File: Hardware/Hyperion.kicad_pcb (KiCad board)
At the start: 2 copper layers, 90.2 x 95.9 mm, 14 parts, among them J1 CUBESAT-BUS, U1 TM4C123GH6PZ

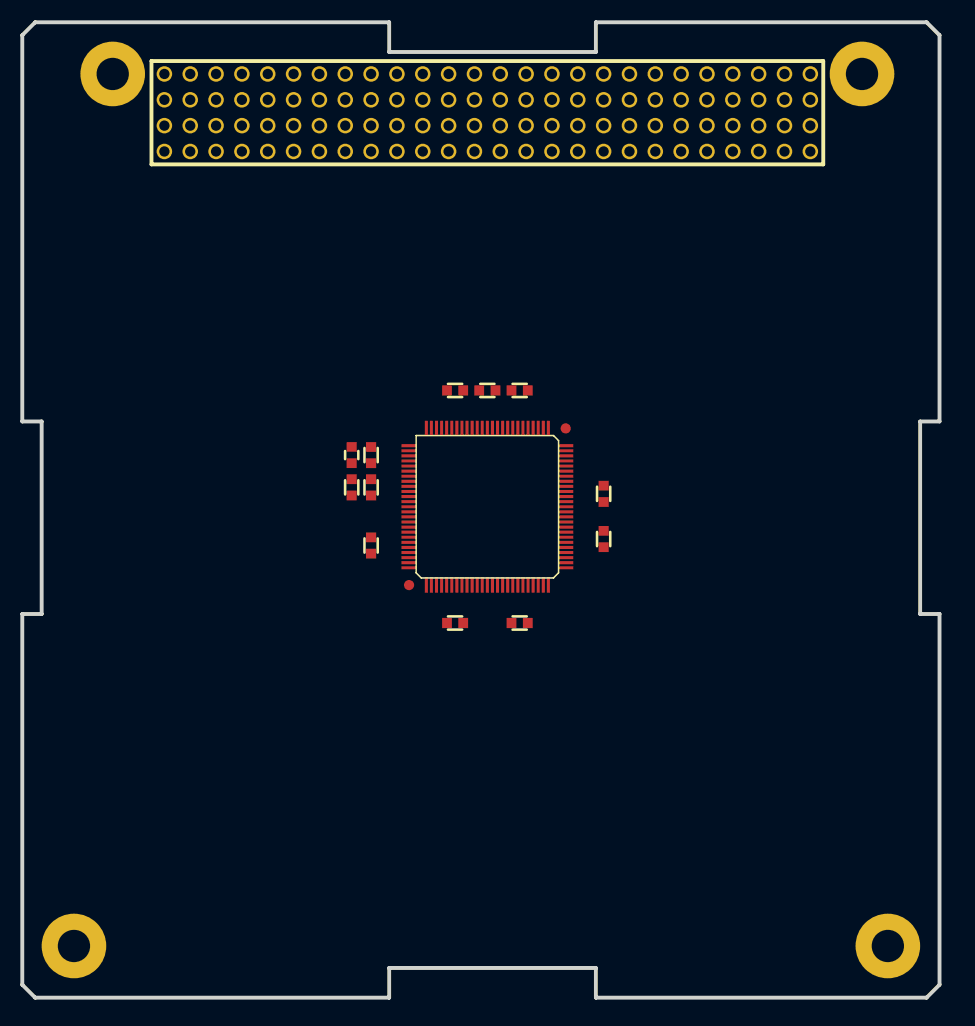
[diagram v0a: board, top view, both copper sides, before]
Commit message: Core layout
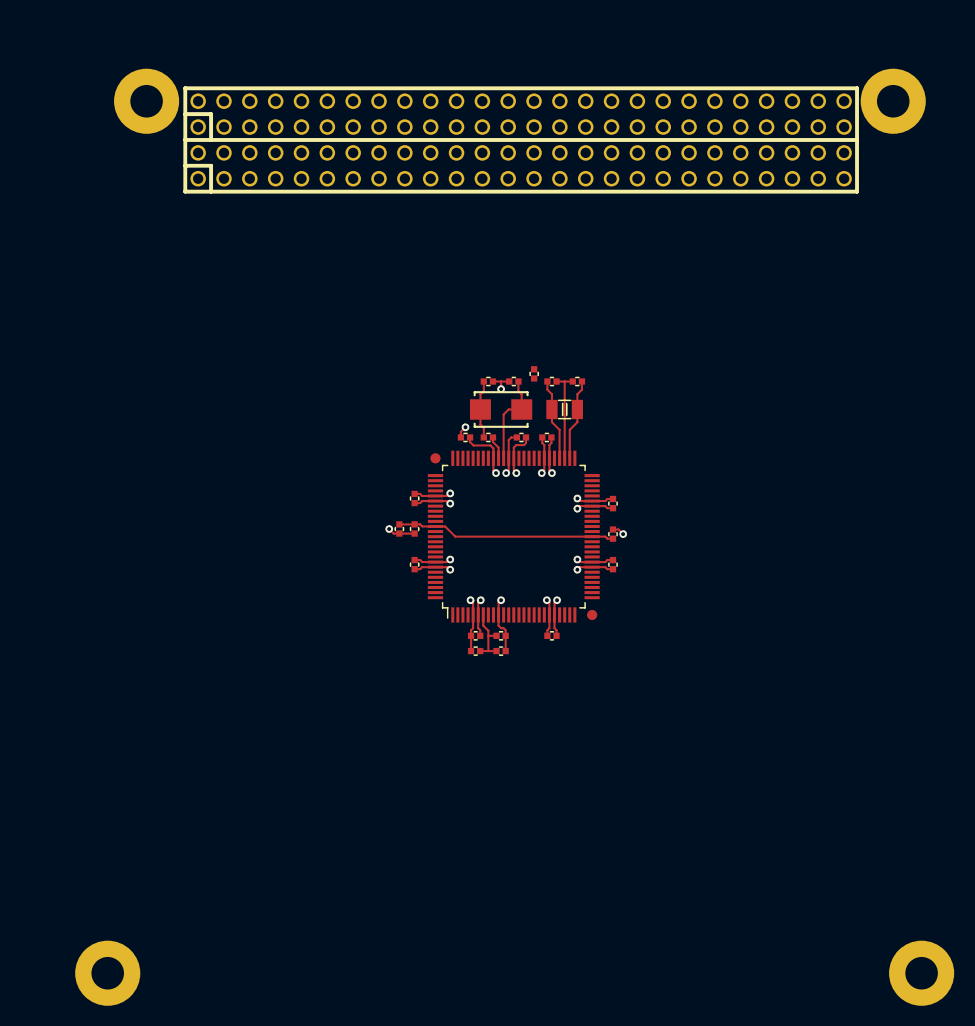
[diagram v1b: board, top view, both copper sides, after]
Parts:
- added C12: 0.1uF, CAPC1005-N, F.Cu at (153.8, 113.2)
- added C13: 0.1uF, CAPC1005-N, F.Cu at (158.2, 92.2)
- added C14: 0.1uF, CAPC1005-N, F.Cu at (150.2, 92.2)
- added C15: C, CAPC1005-N, F.Cu at (155.0, 86.8)
- added C16: 0.1uF, CAPC1005-N, F.Cu at (145.2, 98.2)
- added C17: C, CAPC1005-N, F.Cu at (152.5, 86.8)
- added C18: 0.1uF, CAPC1005-N, F.Cu at (145.2, 104.8)
- added R1: 1k, RESC1005-N, F.Cu at (157.0, 86.0)
- added R2: R, RESC1005-N, F.Cu at (152.5, 92.2)
- added X1: 32.768kHz, XTAL-2SMD-32x15, F.Cu at (160.0, 89.5)
- added X2: 16MHz, XTAL-2SMD-50X32, F.Cu at (153.8, 89.5)
- C1: value 3.3uF -> 0.1uF; footprint CAPC1608 -> CAPC1005-N
- C10: value 1000pF -> 0.1uF; footprint CAPC1608 -> CAPC1005-N
- C11, C8: value 0.1uF -> 20pF; footprint CAPC1608 -> CAPC1005-N
- C2, C3, C4, C5, C7: footprint CAPC1608 -> CAPC1005-N
- C6: value 0.1uF -> 3.3uF; footprint CAPC1608 -> CAPC1005-N
- C9: value 0.1uF -> 1000pF; footprint CAPC1608 -> CAPC1005-N
- FB1: footprint INDC1608 -> INDC1005-N
- moved C9 24.5 mm to (153.8, 111.8), turned to 0 degrees
- moved C10 23.8 mm to (164.8, 98.8), turned to 90 degrees
- moved FB1 22.8 mm to (151.2, 113.2), turned to 180 degrees
- moved C11 22.3 mm to (158.8, 86.8), turned to 0 degrees
- moved C2 20.5 mm to (151.2, 111.8), turned to 0 degrees
- moved C6 20.1 mm to (143.8, 101.2), turned to 270 degrees
- moved C1 18.8 mm to (164.8, 101.8), turned to 90 degrees
- moved C3 18.2 mm to (155.8, 92.2), turned to 180 degrees
- moved C4 10.1 mm to (145.2, 101.2), turned to 270 degrees
- moved C7 7.02 mm to (164.8, 104.8), turned to 90 degrees
- moved C8 5.74 mm to (161.2, 86.8)
- moved J1 4.27 mm to (110.0, 150.0)
- moved U1 3.92 mm to (155.0, 102.0)
- moved C5 3.42 mm to (158.8, 111.8)
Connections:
- C1 pad 1: N-00000105 -> N-00000153
- C10 pad 1: N-00000109 -> +3.3VDAC
- C10 pad 2: GNDA -> GND
- C11 pad 1: N-00000109 -> /Core/XOSC1
- C11 pad 2: GNDA -> /Core/GNDX
- C2 pad 1: +3.3V -> +3.3VDAC
- C3 pad 1: +3.3V -> /Core/~RST
- C4 pad 1: +3.3V -> N-00000153
- C5 pad 1: +3.3V -> +3.3VDAC
- C6 pad 1: +3.3V -> N-00000153
- C7 pad 1: +3.3V -> +3.3VDAC
- C8 pad 1: +3.3V -> /Core/XOSC0
- C8 pad 2: GND -> /Core/GNDX
- C9 pad 1: +3.3V -> +3.3VADC
- FB1 pad 1: N-00000109 -> +3.3VADC
- FB1 pad 2: +3.3V -> +3.3VDAC
- J1 pad 2.25: (no net) -> +5V
- J1 pad 2.26: (no net) -> +5V
- J1 pad 2.27: (no net) -> +3.3V
- J1 pad 2.28: (no net) -> +3.3V
- J1 pad 2.29: (no net) -> DGND
- J1 pad 2.30: (no net) -> DGND
- J1 pad 2.32: (no net) -> DGND
- J1 pad 2.45: (no net) -> +BATT
- J1 pad 2.46: (no net) -> +BATT
- U1 pad 10: GNDA -> GND
- U1 pad 20: +3.3V -> +3.3VDAC
- U1 pad 32: +3.3V -> +3.3VDAC
- U1 pad 38: N-00000105 -> N-00000153
- U1 pad 44: +3.3V -> +3.3VDAC
- U1 pad 5: +3.3V -> +3.3VDAC
- U1 pad 52: (no net) -> /Core/XOSC0
- U1 pad 53: (no net) -> /Core/GNDX
- U1 pad 54: (no net) -> /Core/XOSC1
- U1 pad 56: +3.3V -> +3.3VDAC
- U1 pad 63: (no net) -> /Core/~RST
- U1 pad 65: (no net) -> /Core/OSC0
- U1 pad 66: (no net) -> /Core/OSC1
- U1 pad 67: +3.3V -> +3.3VDAC
- U1 pad 7: N-00000109 -> +3.3VADC
- U1 pad 80: +3.3V -> +3.3VDAC
- U1 pad 82: (no net) -> /Core/TDO
- U1 pad 83: (no net) -> /Core/TDI
- U1 pad 84: (no net) -> /Core/TMS
- U1 pad 85: (no net) -> /Core/TCK
- U1 pad 86: N-00000105 -> N-00000153
- U1 pad 93: +3.3V -> +3.3VDAC
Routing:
- net GND: track 0.00 -> 43.0 mm, vias 0 -> 13
- net +3.3VDAC: track 0.00 -> 32.8 mm, vias 0 -> 8
- net N-00000153: track 0.00 -> 21.6 mm
- net /Core/OSC0: track 0.00 -> 9.17 mm
- net /Core/GNDX: track 0.00 -> 9.15 mm
- net /Core/XOSC1: track 0.00 -> 8.05 mm
- net /Core/XOSC0: track 0.00 -> 8.05 mm
- net +3.3VADC: track 0.00 -> 6.16 mm
- net N-0000089: track 0.00 -> 5.77 mm
- net /Core/~RST: track 0.00 -> 4.54 mm, vias 0 -> 1
- net /Core/OSC1: track 0.00 -> 2.28 mm
- added copper zone on Inner2.Cu, net +3.3VDAC
- added copper zone on Inner1.Cu, net GND
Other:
- board outline removed
- copper layers 2 -> 4
- net class Default: clearance 0.254 -> 0.2032; trace_width 0.254 -> 0.2032; via_dia 0.889 -> 0.762; via_drill 0.635 -> 0.381
- rule trace_clearance: 0.254 -> 0.2032
- rule trace_min: 0.254 -> 0.2032
- rule via_min_drill: 0.508 -> 0.381
- rule via_min_size: 0.889 -> 0.635
